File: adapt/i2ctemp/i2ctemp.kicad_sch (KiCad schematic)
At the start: 9 parts

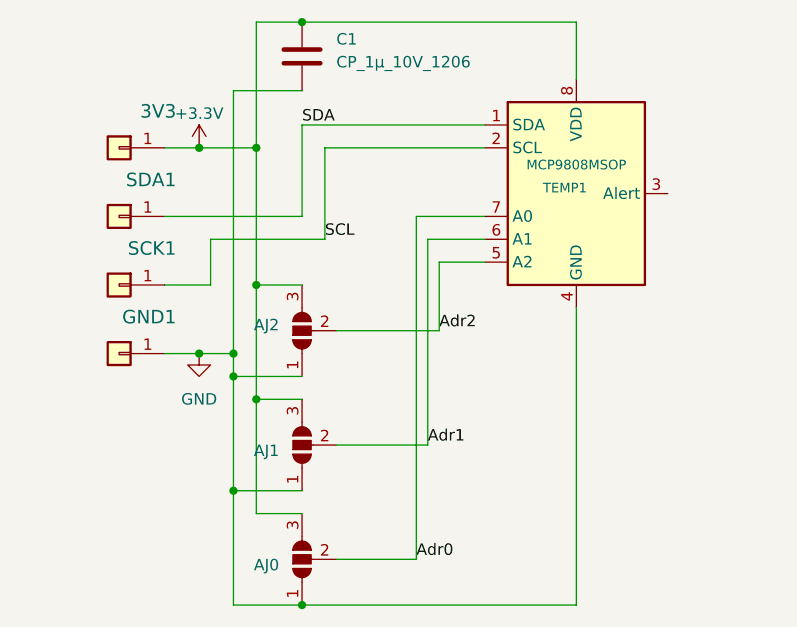
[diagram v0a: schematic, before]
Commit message: Old check-in: i2ctemp
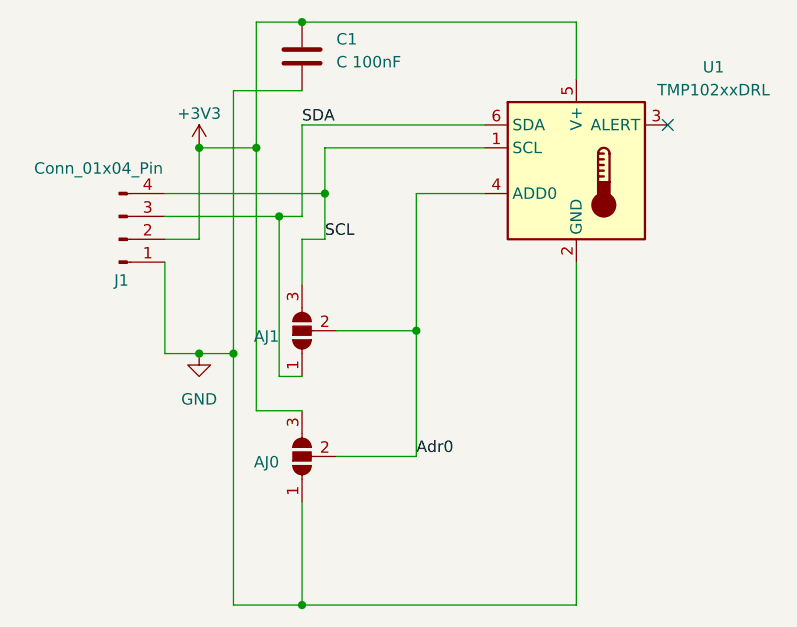
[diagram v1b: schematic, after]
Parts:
- removed 3V3, GND1, SCK1, SDA1: PINHD-1X1CB, i2ctemp:1X01-CLEANBIG, symbol Connector_Generic:Conn_01x01
- removed AJ2: SolderJumper_3_Open, symbol Jumper:SolderJumper_3_Open
- removed TEMP1: MCP9808MSOP, Package_SO:MSOP-8_3x3mm_P0.65mm, symbol localstuff:MCP9808_MSOP
- added J1: Conn_01x04_Pin, Connector_JST:JST_SH_SM04B-SRSS-TB_1x04-1MP_P1.00mm_Horizontal, symbol Connector:Conn_01x04_Pin
- added U1: TMP102xxDRL, Package_TO_SOT_SMD:SOT-563, symbol Sensor_Temperature:TMP102xxDRL
- AJ0, AJ1: now left out of the parts list
- C1: value CP_1µ_10V_1206 -> C 100nF; footprint Resistor_SMD:R_1206_3216Metric_Pad1.30x1.75mm_HandSolder -> Capacitor_SMD:C_0402_1005Metric; LCSC (none) -> C22435938
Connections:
- net Adr1 is gone; now on net Adr0: AJ1.2 (C)
- net +3V3: now also J1.2 (Pin_2), U1.5 (V+); no longer AJ1.3 (B)
- net Adr0: now also U1.4 (ADD0)
- net GND: now also J1.1 (Pin_1), U1.2 (GND); no longer AJ1.1 (A)
- net SCL: now also AJ1.3 (B), J1.4 (Pin_4), U1.1 (SCL)
- net SDA: now also AJ1.1 (A), J1.3 (Pin_3), U1.6 (SDA)
- no-connect marks 0 -> 1
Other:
- moved on the sheet: AJ0, AJ1
